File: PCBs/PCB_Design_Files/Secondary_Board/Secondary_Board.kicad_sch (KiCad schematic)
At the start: 6 parts, among them J1 Conn_FFC_8pin, J2 Conn_01x08_Pin

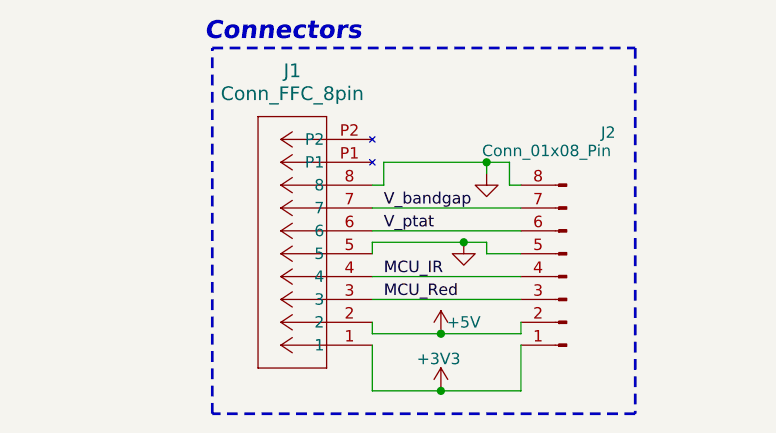
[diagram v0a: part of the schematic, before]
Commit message: LED Driver Updates
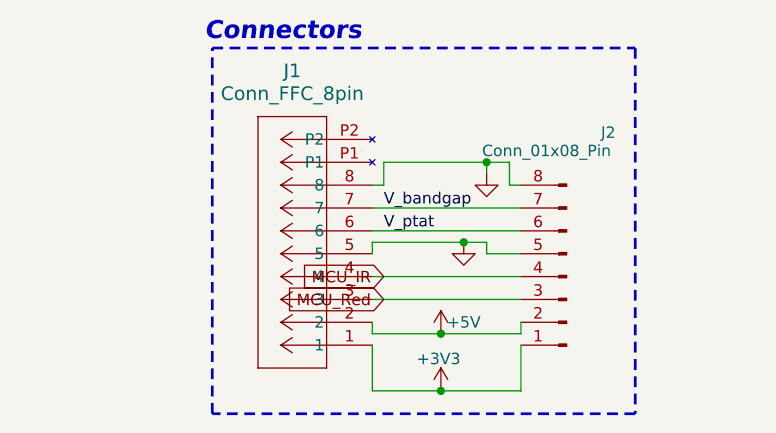
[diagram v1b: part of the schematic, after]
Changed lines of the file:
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@@
-		)
-	)
-	(label "MCU_IR"
-		(at 41.91 113.03 0)
-		(effects
-			(font
-				(size 1.27 1.27)
-			)
-			(justify left bottom)
 		)
 	)
@@
 		)
 	)
-	(label "MCU_Red"
-		(at 41.91 115.57 0)
+	(global_label "MCU_IR"
+		(shape input)
+		(at 41.91 113.03 180)
+		(fields_autoplaced yes)
 		(effects
 			(font
 				(size 1.27 1.27)
 			)
-			(justify left bottom)
+			(justify right)
+		)
+		(property "Intersheetrefs" "${INTERSHEET_REFS}"
+			(at 32.0305 113.03 0)
+			(effects
+				(font
+					(size 1.27 1.27)
+				)
+				(justify right)
+				(hide yes)
+			)
 		)
 	)
+	(global_label "MCU_Red"
+		(shape input)
+		(at 41.91 115.57 180)
+		(fields_autoplaced yes)
+		(effects
+			(font
+				(size 1.27 1.27)
+			)
+			(justify right)
+		)
+		(property "Intersheetrefs" "${INTERSHEET_REFS}"
+			(at 30.3977 115.57 0)
+			(effects
+				(font
+					(size 1.27 1.27)
+				)
+				(justify right)
+				(hide yes)
+			)
+		)
+	)
